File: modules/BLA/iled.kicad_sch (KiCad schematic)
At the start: 3 parts

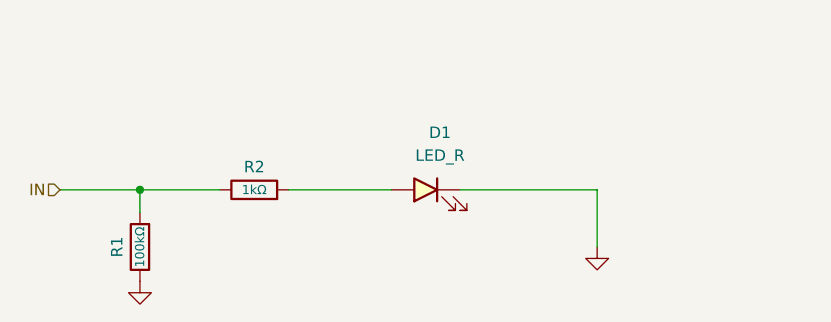
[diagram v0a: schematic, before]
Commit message: minor PW PCB tweaks
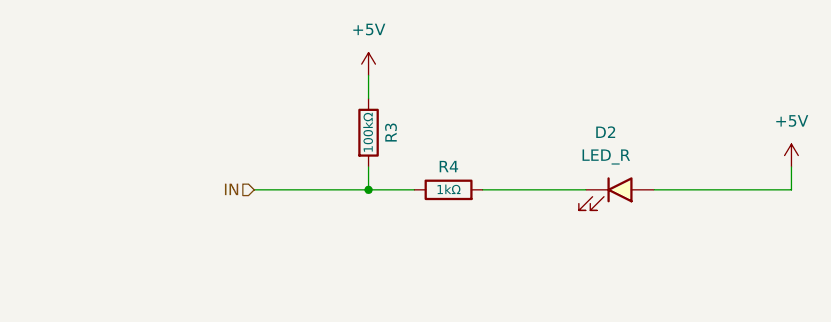
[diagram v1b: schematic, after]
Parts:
- removed D1: LED_R, LED_THT:LED_D3.0mm_Horizontal_O1.27mm_Z2.0mm, symbol IMNOTWOPR:LED_R
- removed R1: 100kΩ, IMNOTWOPR:R_Axial_DIN0207_P400mil, symbol IMNOTWOPR:R
- removed R2: 1kΩ, IMNOTWOPR:R_Axial_DIN0207_P400mil, symbol IMNOTWOPR:R
- added D2: LED_R, LED_THT:LED_D3.0mm_Horizontal_O1.27mm_Z2.0mm, symbol IMNOTWOPR:LED_R
- added R3: 100kΩ, IMNOTWOPR:R_Axial_DIN0207_P400mil, symbol IMNOTWOPR:R
- added R4: 1kΩ, IMNOTWOPR:R_Axial_DIN0207_P400mil, symbol IMNOTWOPR:R
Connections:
- net IN: now also R3.2, R4.1
- new net: D2.1 (K), R4.2
- new net +5V: D2.2 (A), R3.1
